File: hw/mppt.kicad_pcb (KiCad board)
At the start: 4 copper layers, 100 x 55 mm, 88 parts, among them J201 1935776, J202 BNC, J301 1935776, J302 1935776, J401 BNC, Q301 SW_L, Q302 SW_H, SW201 SW_Push, U201 MCU_Nucleo_L432KC, U401 OPA990, U402 INA210, U403 OPA990, U404 INA210, U501 LMG1210RVRT

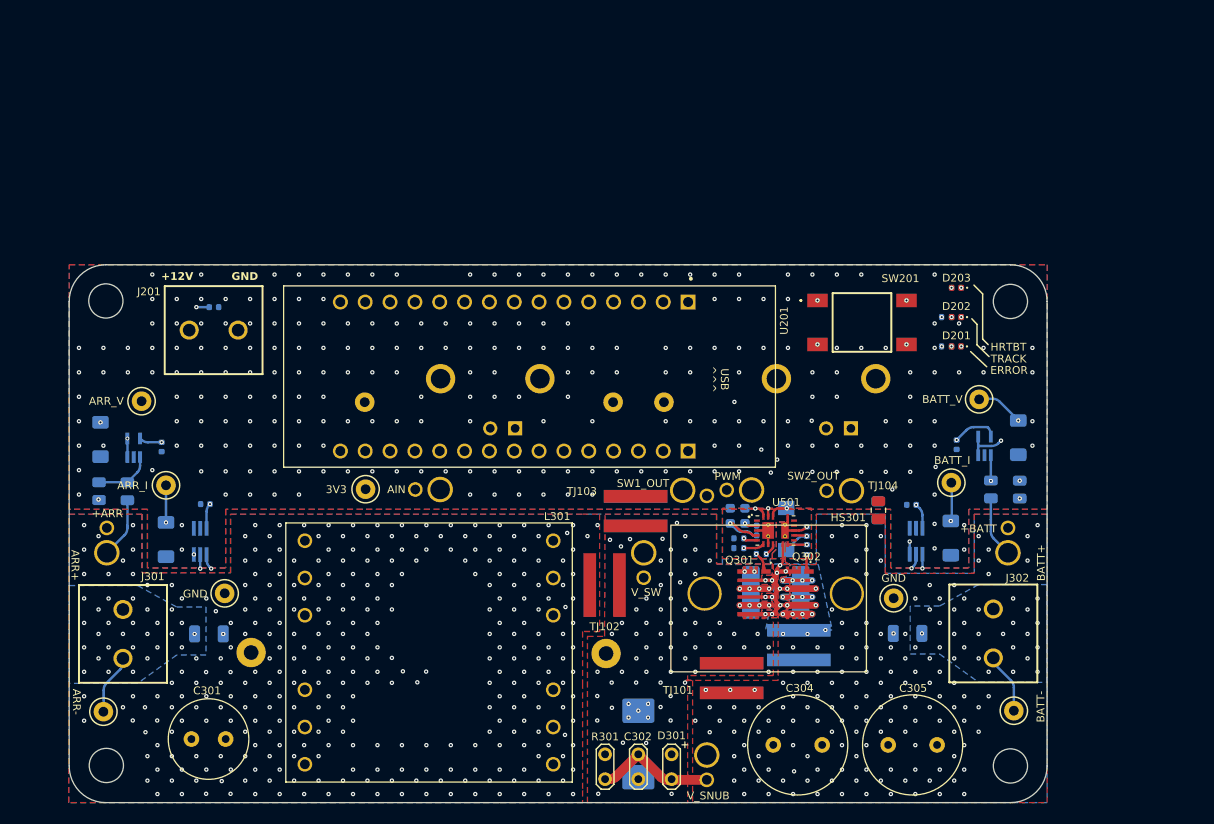
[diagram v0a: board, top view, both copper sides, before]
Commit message: v0.2.0
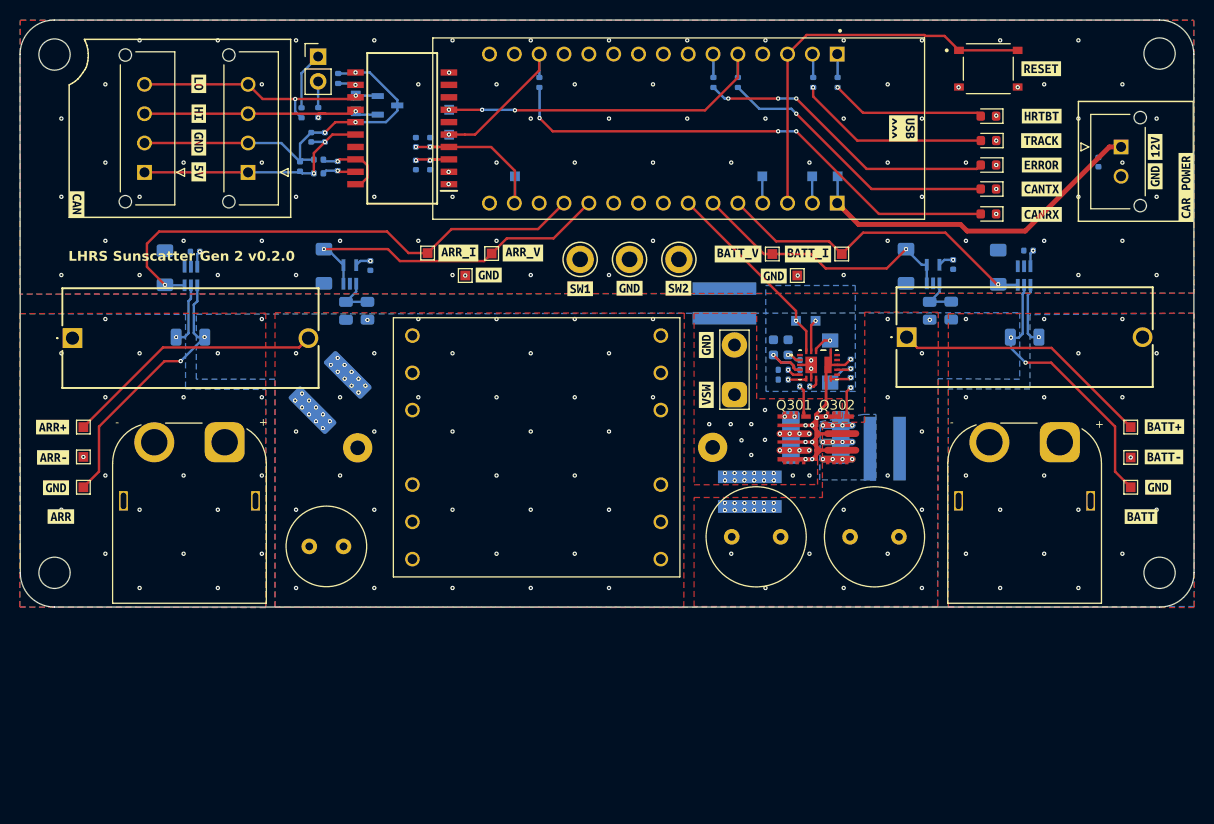
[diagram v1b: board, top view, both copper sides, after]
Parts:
- removed D301: Schottky, TestPoint:TestPoint_2Pads_Pitch2.54mm_Drill0.8mm
- removed D302: D_TVS, Diode_SMD:D_SMC
- removed G***: LOGO, graphics:Texas Engineering
- removed HS301: Heatsink_Pad, mppt:WayinTop_HS
- removed J202, J401: BNC, mppt:CONBNC002
- removed R301: R, TestPoint:TestPoint_2Pads_Pitch2.54mm_Drill0.8mm
- removed the REF** at (128.2, 97.0)
- removed SW201: SW_Push, mppt:TS046643BK100SMT
- removed TJ104, TJ105: Thermal Jumper, Resistor_SMD:R_0805_2012Metric
- removed TJ106, TJ107: Thermal Jumper, mppt:1225_SMD
- removed TP205: GND MCU TP, TestPoint:TestPoint_Keystone_5000-5004_Miniature
- removed TP302: TestPoint_2Pole, mppt:SignalTP
- removed U401, U403: OPA990, mppt:SOT65P210X110-5N
- removed U402, U404: INA210, Package_TO_SOT_SMD:SOT-363_SC-70-6_Handsoldering
- removed U501: LMG1210RVRT, mppt:IC_LMG1210RVRT
- added C601: 10uF, Capacitor_SMD:C_0402_1005Metric, B.Cu at (125.5, 54.8)
- added C602: 100nF, Capacitor_SMD:C_0402_1005Metric, B.Cu at (126.9, 54.8)
- added C603: 100nF, Capacitor_SMD:C_0402_1005Metric, B.Cu at (125.5, 52.5)
- added C604: 10nF, Capacitor_SMD:C_0402_1005Metric, B.Cu at (126.9, 52.5)
- added C605: 220nF, Capacitor_SMD:C_0402_1005Metric, B.Cu at (117.5, 54.9)
- added C606: 10uF, Capacitor_SMD:C_0402_1005Metric, B.Cu at (113.6, 55.0)
- added C607: 10nF, Capacitor_SMD:C_0402_1005Metric, B.Cu at (116.2, 52.0)
- added C608: 100nF, Capacitor_SMD:C_0402_1005Metric, B.Cu at (114.8, 52.0)
- added D204: BLUE, LED_SMD:LED_0603_1608Metric, F.Cu at (184.0, 57.2)
- added D205: BLUE, LED_SMD:LED_0603_1608Metric, F.Cu at (184.0, 59.8)
- added D601: CDSOT23-T24CAN, footprints:bourns_CDSOT23_T24CAN, B.Cu at (122.6, 48.7)
- added F301: Fuse_Small, footprints:littelfuse_05200101Z, F.Cu at (90.3, 72.5)
- added F302: Fuse_Small, footprints:littelfuse_05200101Z, F.Cu at (175.6, 72.4)
- added IC401: INA210CQDCKRQ1, footprints:ti_INA210CQDCKRQ1, B.Cu at (102.5, 66.2)
- added IC402: OPA990IDCKR, footprints:ti_OPA990IDCKR, B.Cu at (118.7, 66.0)
- added IC403: OPA990IDCKR, footprints:ti_OPA990IDCKR, B.Cu at (178.3, 66.0)
- added IC404: INA210CQDCKRQ1, footprints:ti_INA210CQDCKRQ1, B.Cu at (187.7, 66.1)
- added IC501: LMG1210RVRT, footprints:ti_LMG1210RVRT, F.Cu at (166.6, 75.2)
- added IC601: ADM3055EBRIZ, footprints:analog_ADM3055EBRIZ, F.Cu at (124.1, 51.0)
- added J601: 43650-0427, footprints:molex_microfit_43650_0427, F.Cu at (97.7, 55.5)
- added J602: 43650-0427, footprints:molex_microfit_43650_0427, F.Cu at (108.3, 55.5)
- added JP601: Termination Resistors, Connector_PinHeader_2.54mm:PinHeader_1x02_P2.54mm_Vertical, F.Cu at (115.5, 43.7)
- added L601: 1.8k, Inductor_SMD:L_0402_1005Metric, B.Cu at (115.5, 55.6)
- added L602: 1.8k, Inductor_SMD:L_0402_1005Metric, B.Cu at (115.5, 54.2)
- added R203: 100, Resistor_SMD:R_0402_1005Metric, B.Cu at (168.6, 46.4)
- added R204: 100, Resistor_SMD:R_0402_1005Metric, B.Cu at (158.4, 46.4)
- added R205: 100, Resistor_SMD:R_0402_1005Metric, B.Cu at (138.1, 46.4)
- added R601: 0, Resistor_SMD:R_0402_1005Metric, B.Cu at (117.5, 46.0)
- added R602: 60.4, Resistor_SMD:R_0402_1005Metric, B.Cu at (115.5, 49.4)
- added R603: 60.4, Resistor_SMD:R_0402_1005Metric, B.Cu at (113.8, 49.5)
- added REF**: ESD-Logo_6.6x6mm_SilkScreen, Symbol:ESD-Logo_6.6x6mm_SilkScreen, B.Cu at (131.1, 91.0)
- added S201: TS-1187A-B-A-B, footprints:xkb_TS_1187A_B_A_B, F.Cu at (184.0, 45.0)
- added TP411: BATTV_TP, TestPoint:TestPoint_Pad_1.0x1.0mm, F.Cu at (161.9, 63.9)
- added TP412: BATTI_TP, TestPoint:TestPoint_Pad_1.0x1.0mm, F.Cu at (169.0, 63.9)
- added TP504: PWMEN_TP, TestPoint:TestPoint_Pad_1.0x1.0mm, B.Cu at (166.3, 70.7)
- added TP505: PWM_TP, TestPoint:TestPoint_Pad_1.0x1.0mm, B.Cu at (164.3, 70.7)
- added TP601: CAN RX TP, TestPoint:TestPoint_Pad_1.0x1.0mm, B.Cu at (128.9, 51.7)
- added TP602: CAN TX TP, TestPoint:TestPoint_Pad_1.0x1.0mm, B.Cu at (128.9, 49.1)
- added TP603: CAN L TP, TestPoint:TestPoint_Pad_1.0x1.0mm, B.Cu at (119.3, 47.7)
- added TP604: CAN H TP, TestPoint:TestPoint_Pad_1.0x1.0mm, B.Cu at (119.3, 49.3)
- added kibuzzard-64BB9525: G***, kibuzzard-64BB9525, F.Cu at (189.4, 52.3)
- added kibuzzard-64BB9530: G***, kibuzzard-64BB9530, F.Cu at (189.4, 49.8)
- added kibuzzard-64BB9539: G***, kibuzzard-64BB9539, F.Cu at (189.4, 54.8)
- added kibuzzard-64BB9548: G***, kibuzzard-64BB9548, F.Cu at (189.4, 59.9)
- added kibuzzard-64BB954F: G***, kibuzzard-64BB954F, F.Cu at (189.4, 57.2)
- added kibuzzard-64BB9585: G***, kibuzzard-64BB9585, F.Cu at (189.4, 45.0)
- added kibuzzard-64BB95E9: G***, kibuzzard-64BB95E9, F.Cu at (204.2, 57.0)
- added kibuzzard-64BB964A: G***, kibuzzard-64BB964A, F.Cu at (201.1, 53.0)
- added kibuzzard-64BB966B: G***, kibuzzard-64BB966B, F.Cu at (201.1, 56.0)
- added kibuzzard-64BB968B: G***, kibuzzard-64BB968B, F.Cu at (175.3, 51.0)
- added kibuzzard-64BB971E: G***, kibuzzard-64BB971E, F.Cu at (90.8, 58.8)
- added kibuzzard-64BB973A: G***, kibuzzard-64BB973A, F.Cu at (103.2, 46.5)
- added kibuzzard-64BB974F: G***, kibuzzard-64BB974F, F.Cu at (103.2, 49.5)
- added kibuzzard-64BB975A: G***, kibuzzard-64BB975A, F.Cu at (103.2, 55.5)
- added kibuzzard-64BB9776: G***, kibuzzard-64BB9776, F.Cu at (103.2, 52.5)
- added kibuzzard-64BB97BE: G***, kibuzzard-64BB97BE, F.Cu at (89.2, 90.8)
- added kibuzzard-64BB97CA: G***, kibuzzard-64BB97CA, F.Cu at (199.6, 90.8)
- added kibuzzard-64BB97F0: G***, kibuzzard-64BB97F0, B.Cu at (106.0, 98.3)
- added kibuzzard-64BB97F0: G***, kibuzzard-64BB97F0, B.Cu at (191.3, 98.2)
- added kibuzzard-64BB97FE: G***, kibuzzard-64BB97FE, B.Cu at (183.9, 98.1)
- added kibuzzard-64BB97FE: G***, kibuzzard-64BB97FE, B.Cu at (98.7, 98.3)
- added kibuzzard-64BB9873: G***, kibuzzard-64BB9873, F.Cu at (88.7, 87.8)
- added kibuzzard-64BB9873: G***, kibuzzard-64BB9873, F.Cu at (201.3, 87.8)
- added kibuzzard-64BB98F2: G***, kibuzzard-64BB98F2, F.Cu at (88.3, 81.6)
- added kibuzzard-64BB98F8: G***, kibuzzard-64BB98F8, F.Cu at (88.3, 84.7)
- added kibuzzard-64BB9946: G***, kibuzzard-64BB9946, F.Cu at (201.9, 84.7)
- added kibuzzard-64BB994C: G***, kibuzzard-64BB994C, F.Cu at (202.0, 81.5)
- added kibuzzard-64BBA694: G***, kibuzzard-64BBA694, F.Cu at (129.8, 63.8)
- added kibuzzard-64BBA6A3: G***, kibuzzard-64BBA6A3, F.Cu at (136.4, 63.8)
- added kibuzzard-64BBA6B0: G***, kibuzzard-64BBA6B0, F.Cu at (162.1, 66.2)
- added kibuzzard-64BBA6B0: G***, kibuzzard-64BBA6B0, F.Cu at (132.9, 66.0)
- added kibuzzard-64BBA752: G***, kibuzzard-64BBA752, F.Cu at (158.4, 63.9)
- added kibuzzard-64BBA758: G***, kibuzzard-64BBA758, F.Cu at (165.6, 63.9)
- added kibuzzard-64BBA88C: G***, kibuzzard-64BBA88C, B.Cu at (160.9, 54.1)
- added kibuzzard-64BBA896: G***, kibuzzard-64BBA896, B.Cu at (165.7, 54.0)
- added kibuzzard-64BBA8A0: G***, kibuzzard-64BBA8A0, B.Cu at (168.9, 54.0)
- added kibuzzard-64BBA8B2: G***, kibuzzard-64BBA8B2, B.Cu at (138.0, 56.0)
- added kibuzzard-64BBA8C3: G***, kibuzzard-64BBA8C3, B.Cu at (163.9, 68.8)
- added kibuzzard-64BBA8E6: G***, kibuzzard-64BBA8E6, B.Cu at (166.3, 68.8)
- added kibuzzard-64BBA9B6: G***, kibuzzard-64BBA9B6, F.Cu at (142.2, 67.5)
- added kibuzzard-64BBA9C0: G***, kibuzzard-64BBA9C0, F.Cu at (147.3, 67.4)
- added kibuzzard-64BBA9D4: G***, kibuzzard-64BBA9D4, F.Cu at (152.3, 67.4)
- added kibuzzard-64BBAA49: G***, kibuzzard-64BBAA49, F.Cu at (155.2, 78.3)
- added kibuzzard-64BBAA54: G***, kibuzzard-64BBAA54, F.Cu at (155.2, 73.2)
- added kibuzzard-64BC07CB: G***, kibuzzard-64BC07CB, B.Cu at (131.0, 49.1)
- added kibuzzard-64BC07D4: G***, kibuzzard-64BC07D4, B.Cu at (131.0, 51.7)
- added kibuzzard-64BC07E0: G***, kibuzzard-64BC07E0, B.Cu at (117.5, 47.7)
- added kibuzzard-64BC07EC: G***, kibuzzard-64BC07EC, B.Cu at (117.5, 49.3)
- C301: value 15uF -> 2.2uF; footprint Capacitor_THT:C_Radial_D8.0mm_H11.5mm_P3.50mm -> Capacitor_SMD:C_2220_5650Metric; moved to B.Cu
- C302: value CP -> 15uF; footprint TestPoint:TestPoint_2Pads_Pitch2.54mm_Drill0.8mm -> Capacitor_THT:C_Radial_D8.0mm_H11.5mm_P3.50mm
- C503: value 1uF -> 10uF; footprint Capacitor_SMD:C_0402_1005Metric -> Capacitor_SMD:C_0603_1608Metric
- C505: value 10uF -> 1uF; footprint Capacitor_SMD:C_0603_1608Metric -> Capacitor_SMD:C_0402_1005Metric
- D201: value RED -> YELLOW; footprint LED_SMD:LED_0402_1005Metric -> LED_SMD:LED_0603_1608Metric
- D202: value YELLOW -> GREEN; footprint LED_SMD:LED_0402_1005Metric -> LED_SMD:LED_0603_1608Metric
- D203: value BLUE -> GREEN; footprint LED_SMD:LED_0402_1005Metric -> LED_SMD:LED_0603_1608Metric
- D402, D403: value 3.3V Zener -> 3V3
- D501: value 0.62V Schottky -> 0.62V; footprint mppt:SODFL5226X110N -> footprints:stm_STPS1170AF
- H101, H102, H103, H104: footprint MountingHole:MountingHole_3.5mm -> MountingHole:MountingHole_3.2mm_M3
- J201: value 1935776 -> 43650-0227; footprint mppt:1935776 -> footprints:molex_microfit_43650_0227
- J301, J302: value 1935776 -> XT60PW-M; footprint mppt:1935776 -> Connector_AMASS:AMASS_XT60PW-M_1x02_P7.20mm_Horizontal
- L301: footprint mppt:B65878E1012D001 -> footprints:tdk_B65878E1012D001
- Q301, Q302: footprint mppt:EPC2307 -> footprints:epc_EPC2307
- R502: value 20k -> 1.8
- R503: value 1.8 -> 20k
- TJ101, TJ102, TJ103: footprint mppt:1225_SMD -> footprints:vishay_THJP1225ABT1; moved to B.Cu
- TP201: value 5V TP -> 3V3 TP; footprint TestPoint:TestPoint_Keystone_5000-5004_Miniature -> TestPoint:TestPoint_Pad_1.0x1.0mm
- TP202: value 3.3V TP -> 5V TP; footprint TestPoint:TestPoint_Keystone_5000-5004_Miniature -> TestPoint:TestPoint_Pad_1.0x1.0mm; moved to B.Cu
- TP203: value 12V TP -> GND TP; footprint TestPoint:TestPoint_Keystone_5000-5004_Miniature -> TestPoint:TestPoint_Pad_1.0x1.0mm
- TP204: value TestPoint_2Pole -> 12V TP; footprint mppt:SignalTP -> TestPoint:TestPoint_Pad_1.0x1.0mm; moved to B.Cu
- TP301: value TestPoint_2Pole -> VSW_TP; footprint mppt:SignalTP -> TestPoint:TestPoint_2Pads_Pitch5.08mm_Drill1.3mm
- TP401: value TestPoint_2Pole -> +ARR_TP; footprint mppt:SignalTP -> TestPoint:TestPoint_Pad_1.0x1.0mm
- TP402: value GND -> GND_TP; footprint TestPoint:TestPoint_Keystone_5000-5004_Miniature -> TestPoint:TestPoint_Pad_1.0x1.0mm
- TP403: value -ARR -> GND_TP; footprint TestPoint:TestPoint_Keystone_5000-5004_Miniature -> TestPoint:TestPoint_Pad_1.0x1.0mm
- TP404: value Array Current -> -ARR_TP; footprint TestPoint:TestPoint_Keystone_5000-5004_Miniature -> TestPoint:TestPoint_Pad_1.0x1.0mm
- TP405: value Array Voltage -> ARRI_TP; footprint TestPoint:TestPoint_Keystone_5000-5004_Miniature -> TestPoint:TestPoint_Pad_1.0x1.0mm
- TP406: value -BATT -> ARRV_TP; footprint TestPoint:TestPoint_Keystone_5000-5004_Miniature -> TestPoint:TestPoint_Pad_1.0x1.0mm
- TP407: value GND -> +BATT_TP; footprint TestPoint:TestPoint_Keystone_5000-5004_Miniature -> TestPoint:TestPoint_Pad_1.0x1.0mm
- TP408: value Battery Current -> GND_TP; footprint TestPoint:TestPoint_Keystone_5000-5004_Miniature -> TestPoint:TestPoint_Pad_1.0x1.0mm
- TP409: value Battery Voltage -> -BATT_TP; footprint TestPoint:TestPoint_Keystone_5000-5004_Miniature -> TestPoint:TestPoint_Pad_1.0x1.0mm
- TP410: value TestPoint_2Pole -> GND_TP; footprint mppt:SignalTP -> TestPoint:TestPoint_Pad_1.0x1.0mm
- TP501: value TestPoint_2Pole -> SW1_TP; footprint mppt:SignalTP -> TestPoint:TestPoint_Keystone_5005-5009_Compact
- TP502: value TestPoint_2Pole -> GND_TP; footprint mppt:SignalTP -> TestPoint:TestPoint_Keystone_5005-5009_Compact
- TP503: value TestPoint_2Pole -> SW2_TP; footprint mppt:SignalTP -> TestPoint:TestPoint_Keystone_5005-5009_Compact
- U201: value MCU_Nucleo_L432KC -> NUCLEO-L432KC; footprint mppt:MODULE_NUCLEO-L432KC -> footprints:stm_nucleo_L432KC
- moved H101 111.3 mm to (201.5, 96.5)
- moved H102 101.6 mm to (88.5, 96.5)
- moved J201 97.1 mm to (197.6, 53.0), turned to 90 degrees
- moved C201 91.7 mm to (195.2, 54.5), turned to -90 degrees
- moved H104 74.4 mm to (201.5, 43.4)
- moved H103 72.9 mm to (88.5, 43.5)
- moved TP406 71.0 mm to (133.2, 63.9)
- moved TP403 57.9 mm to (130.5, 66.1)
- moved TP204 52.7 mm to (168.6, 56.0), turned to -90 degrees
- moved TP202 51.7 mm to (160.9, 56.0), turned to -90 degrees
- moved TP203 51.3 mm to (166.0, 56.0), turned to -90 degrees
- moved C302 39.8 mm to (114.5, 93.8), turned to 0 degrees
- moved TP301 38.2 mm to (158.0, 78.3), turned to 90 degrees
- moved C301 37.0 mm to (116.7, 78.1), turned to -135 degrees
- moved R201 36.0 mm to (155.9, 46.4), turned to 90 degrees
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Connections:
- C302 pad 1: /converter/Vsnub -> /V_ARR+
- C401 pad 2: +12V -> +5V
- C402 pad 2: +12V -> +5V
- C403 pad 2: +12V -> +5V
- C404 pad 2: +12V -> +5V
- C501 pad 1: +12V -> +5V
- C502 pad 1: +12V -> +5V
- C503 pad 1: /V_SW -> +12V
- C503 pad 2: /gate_driver/HB -> GND
- C504 pad 1: +5V -> +12V
- C505 pad 1: +5V -> Net-(D501-K)
- C505 pad 2: GND -> /V_SW
- D203 pad 2: /controller/Heartbeat -> Net-(D203-A)
- D403 pad 1: /controller/BATT_I -> /controller/BATT_V
- D404 pad 1: /controller/BATT_V -> /controller/BATT_I
- D501 pad 1: /gate_driver/HB -> Net-(D501-K)
- D501 pad 2: /gate_driver/BST -> Net-(D501-A)
- J301 pad 1: /V_ARR+ -> Net-(F301-Pad1)
- J302 pad 1: /V_BATT+ -> Net-(F302-Pad2)
- R501 pad 1: /gate_driver/DLH -> Net-(IC501-DHL)
- R502 pad 1: /gate_driver/DHL -> /converter/G1
- R502 pad 2: GND -> Net-(IC501-LO)
- R503 pad 1: /gate_driver/LO -> GND
- R503 pad 2: /converter/G1 -> Net-(IC501-DLH)
- R504 pad 1: /gate_driver/HO -> /converter/G2
- R504 pad 2: /converter/G2 -> Net-(IC501-HO)
- TJ102 pad 1: /V_SW -> GND
- TJ102 pad 2: /V_ARR+ -> /V_BATT+
- TJ103 pad 1: /V_SW -> GND
- TJ103 pad 2: +12V -> GND
- TP201 pad 1: +5V -> +3V3
- TP202 pad 1: +3.3V -> +5V
- TP203 pad 1: +12V -> GND
- TP204 pad 1: /controller/PWM_CTRL -> +12V
- TP301 pad 1: /converter/Vsnub -> /V_SW
- TP403 pad 1: /converter/V_ARR- -> GND
- TP404 pad 1: /controller/ARR_I -> /converter/V_ARR-
- TP405 pad 1: /controller/ARR_V -> /controller/ARR_I
- TP406 pad 1: /converter/V_BATT- -> /controller/ARR_V
- TP407 pad 1: GND -> /V_BATT+
- TP408 pad 1: /controller/BATT_I -> GND
- TP409 pad 1: /controller/BATT_V -> /converter/V_BATT-
- TP410 pad 1: /V_BATT+ -> GND
- TP501 pad 1: /controller/PWM -> /converter/G1
- TP502 pad 1: /converter/G1 -> GND
- U201 pad 13: unconnected-(U201-D10-Pad13) -> /CAN_RX
- U201 pad 17: +3.3V -> +3V3
- U201 pad 19: /controller/PWM_CTRL -> /controller/ARR_I
- U201 pad 20: /controller/PWM -> /controller/ARR_V
- U201 pad 21: /controller/PWM_EN -> unconnected-(U201-A2-Pad21)
- U201 pad 22: /controller/ARR_V -> unconnected-(U201-A3-Pad22)
- U201 pad 23: /controller/ARR_I -> /controller/PWM_EN
- U201 pad 24: /controller/BATT_I -> /controller/PWM
- U201 pad 26: unconnected-(U201-A7-Pad26) -> /controller/BATT_I
- U201 pad 5: unconnected-(U201-D2-Pad5) -> /CAN_TX
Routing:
- net Net-(D205-A): track 0.00 -> 52.3 mm, vias 0 -> 3
- net +12V: track 18.1 -> 59.8 mm, vias 6 -> 1
- net Net-(D601-K3): track 0.00 -> 39.8 mm, vias 0 -> 3
- net /controller/Error: track 40.4 -> 2.41 mm, vias 1 -> 0
- net /CAN_TX: track 0.00 -> 35.7 mm, vias 0 -> 3
- net /controller/BATT_V: track 62.3 -> 28.0 mm, vias 2 -> 1
- net GND: track 44.5 -> 76.9 mm, vias 522 -> 111
- net Net-(D201-A): track 0.00 -> 31.0 mm, vias 1 -> 3
- net Net-(D204-A): track 0.00 -> 29.1 mm, vias 0 -> 1
- net /comm_can/CAN_L: track 0.00 -> 26.9 mm, vias 0 -> 2
- net /controller/Tracking: track 29.1 -> 2.42 mm, vias 1 -> 0
- net Net-(IC601-VISOIN): track 0.00 -> 26.0 mm, vias 0 -> 2
- net /comm_can/CAN_H: track 0.00 -> 25.4 mm, vias 0 -> 2
- net /controller/Heartbeat: track 27.3 -> 2.41 mm, vias 1 -> 0
- net /V_ARR+: track 3.54 -> 26.8 mm, vias 154 -> 25
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- added copper zone on F.Cu, net +5V
- added copper zone on In1.Cu, net +5V
- added copper zone on F.Cu, net Net-(F301-Pad1)
- added copper zone on In1.Cu, net Net-(F301-Pad1)
- added copper zone on F.Cu, net Net-(F302-Pad2)
- added copper zone on In1.Cu, net Net-(F302-Pad2)
- removed copper zone on F.Cu, net +12V
- removed copper zone on B.Cu, net /V_SW
- removed copper zone on In2.Cu, net /V_SW
- removed copper zone on In1.Cu, net GND
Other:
- board size 100 x 55 mm -> 120.1 x 60 mm
- board text added: "LHR Solar Sunscatter Gen 2 v0.2.0 Summer 2023 Matthew Yu"
- board text added: "LHRS Sunscatter Gen 2 v0.2.0"
- board text added: "Trace should not modify fill. Used to remove DRC."
- board text removed: "+"
- board text removed: "+12V"
- board text removed: "."
- board text removed: "ARR+"
- board text removed: "ARR-"
- board text removed: "BATT+"
- board text removed: "BATT-"
- board text removed: "GND"
- board text removed: "Sunscatter MPPT LHR Solar 2023 Jacob Pustilnik Matthew Yu v0.1.1"
- board text removed: "USB ^^^"
